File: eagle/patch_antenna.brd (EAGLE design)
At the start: 203.2 x 203.2 mm, 2 parts

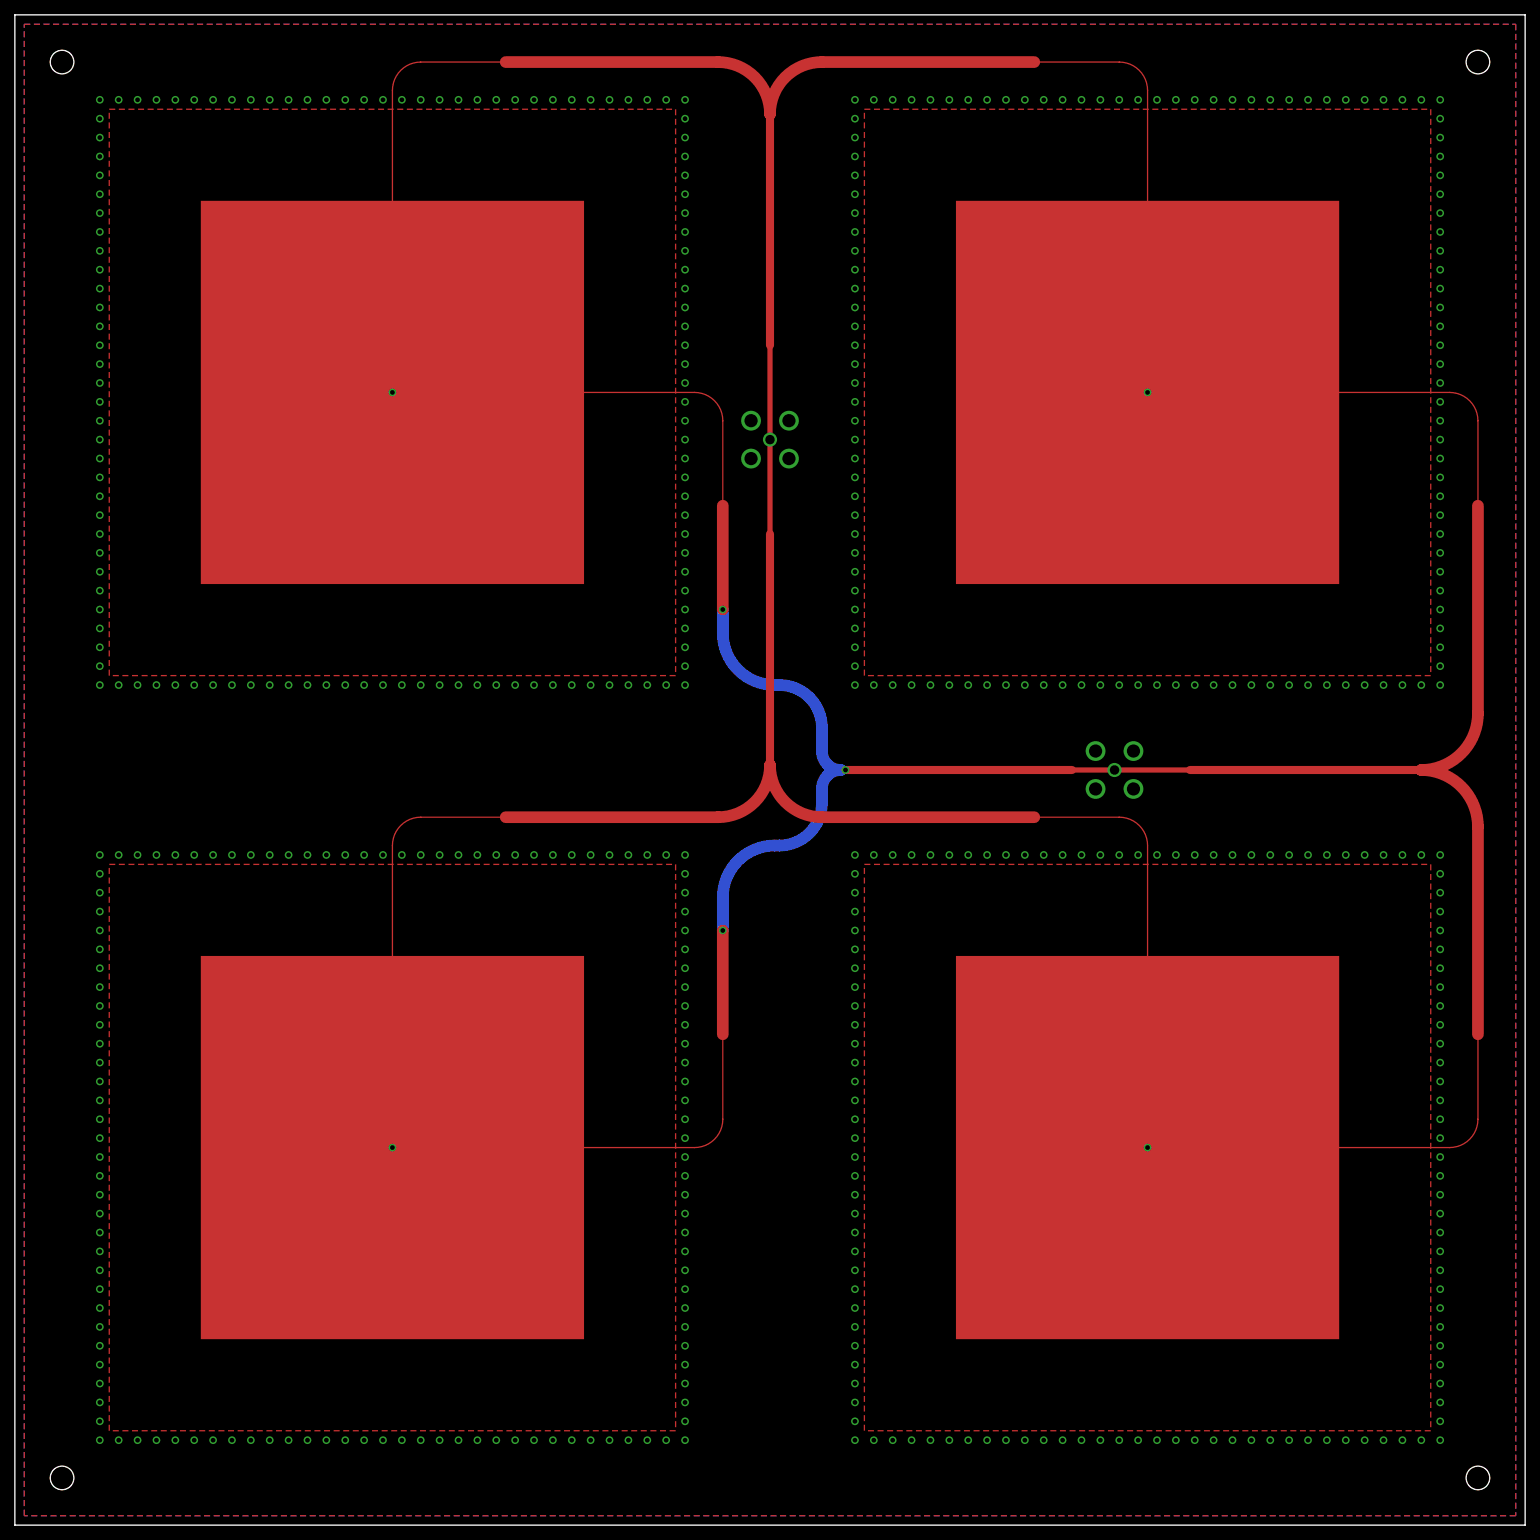
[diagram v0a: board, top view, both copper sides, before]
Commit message: reorganize eagle files
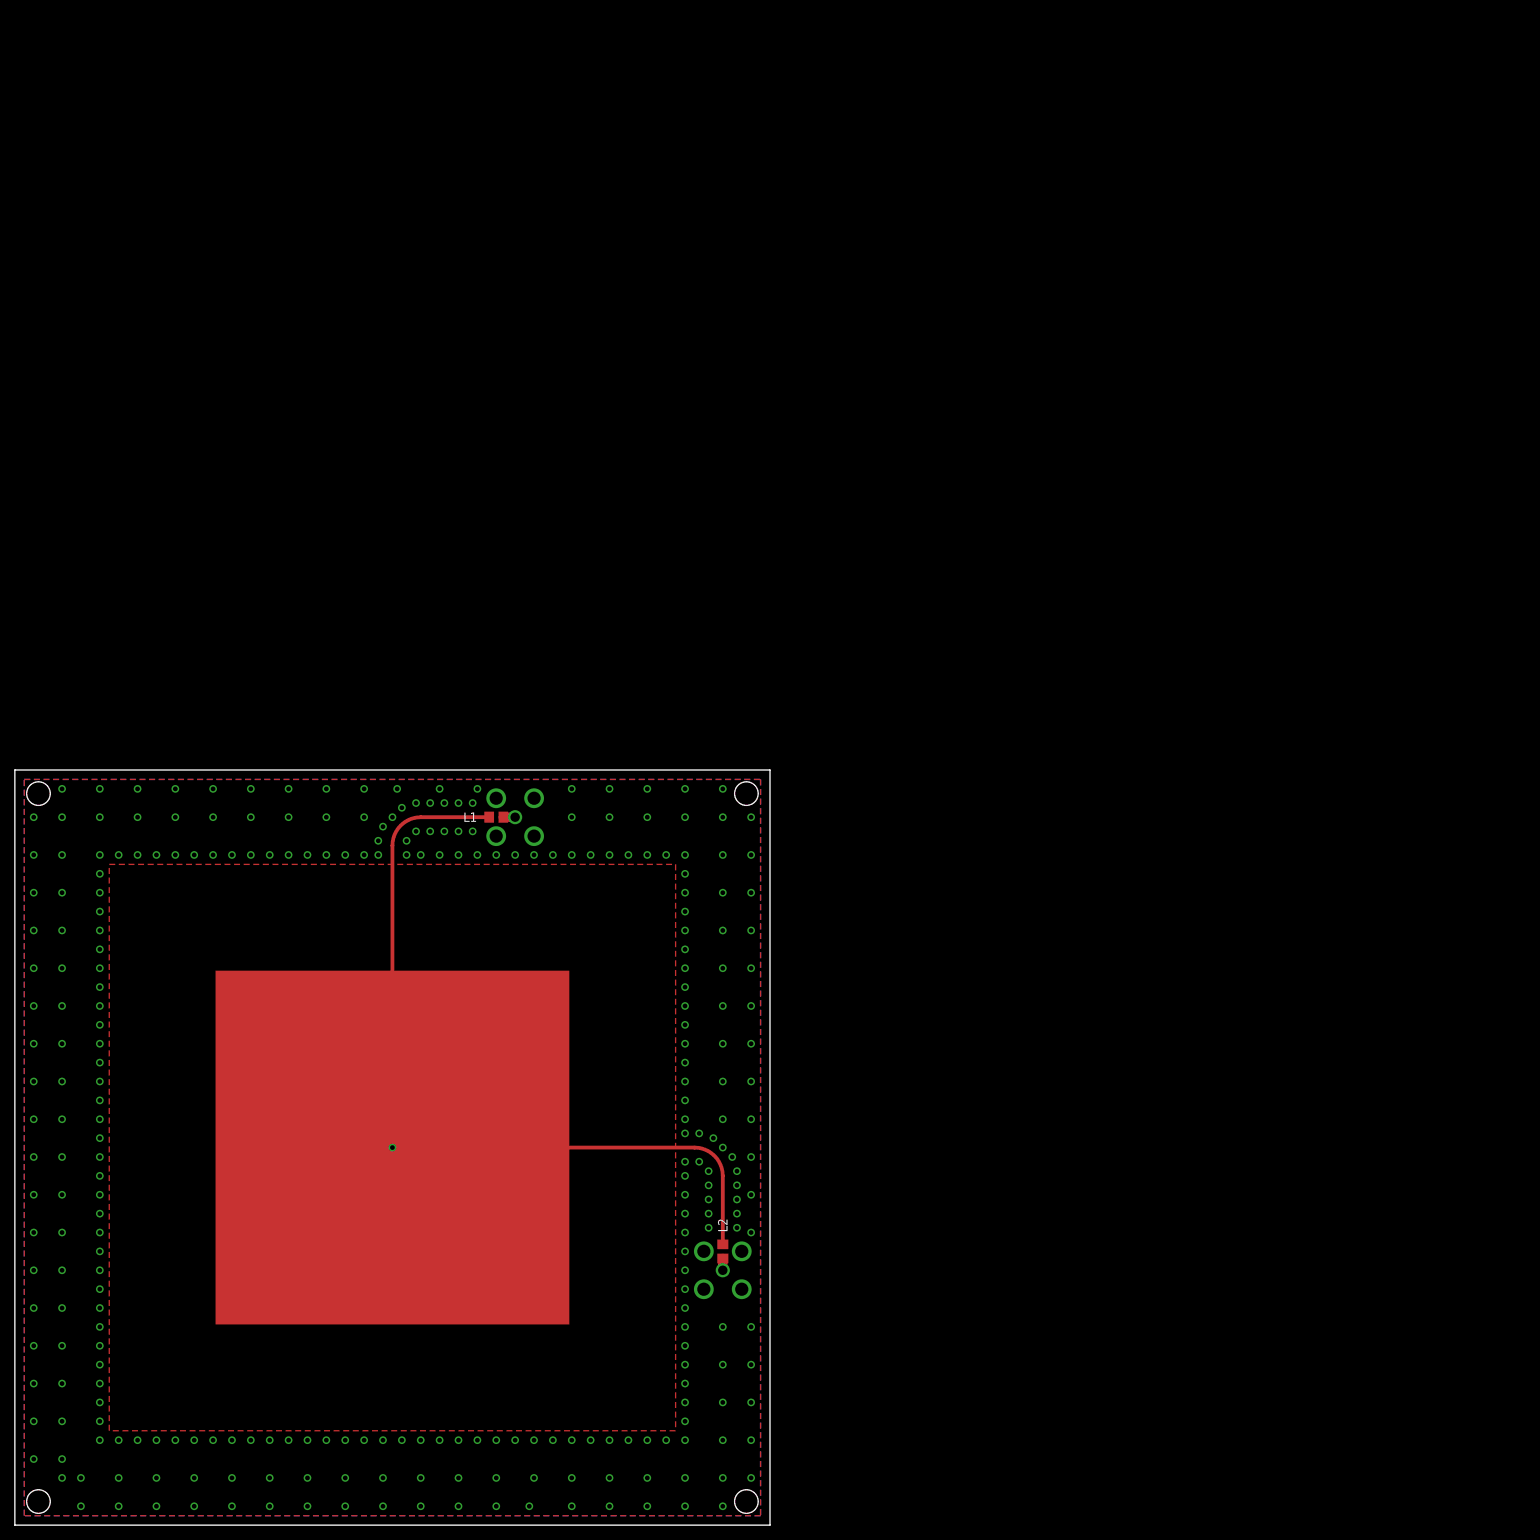
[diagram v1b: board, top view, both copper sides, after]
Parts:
- added L1, L2: 2.7n, rcl:C0805
- moved J1 111.9 mm to (95.2, 34.3)
- moved J2 80.9 mm to (67.3, 95.2)
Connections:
- removed net H: J2.1
- removed net V: J1.1
- new net S$1: J2.1, L1.2
- new net S$2: J1.1, L2.2
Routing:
- net V: track 371.5 -> 31.1 mm
- net H: track 369.0 -> 31.1 mm, vias 3 -> 0
- net S$2: track 0.00 -> 1.59 mm
- net S$1: track 0.00 -> 1.59 mm
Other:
- board size 203.2 x 203.2 mm -> 101.6 x 101.6 mm
